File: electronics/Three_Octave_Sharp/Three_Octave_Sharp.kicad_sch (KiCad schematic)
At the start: 107 parts, among them J1 HRO_TYPE-C-31-M-12, SW1 Key Tab, SW10 Key O, SW11 Key P, SW12 Key BS, SW16 Key Caps, SW17 Key A, SW18 Key S, SW19 Key D, SW2 Key Q, SW20 Key F, SW21 Alps_Alpine_SKRP, SW21 Key G, SW22 Alps_Alpine_SKRP, SW22 Key H, SW23 Key J, SW24 Key K, SW25 Key L, SW26 Key Return, SW3 Key W, SW30 Key Shift, SW31 Key Z, SW32 Key X, SW33 Key C, SW33 Key Shift, SW34 Key V, SW35 Key B, SW36 Key N, SW37 Key M, SW38 Key ,, SW4 Key E, SW43 Key Ctrl, SW44 Key Cmd, SW45 Key Space, SW46 Key Opt, SW47 Key Fn, SW5 Key R, SW6 Key T, SW7 Key Y, SW8 Key U, SW9 Key I, U1 AP2112K-3.3, U2 Raspberry_Pi_RP2040, U2 W25Q64JVXGIQ, Y1 12MHz

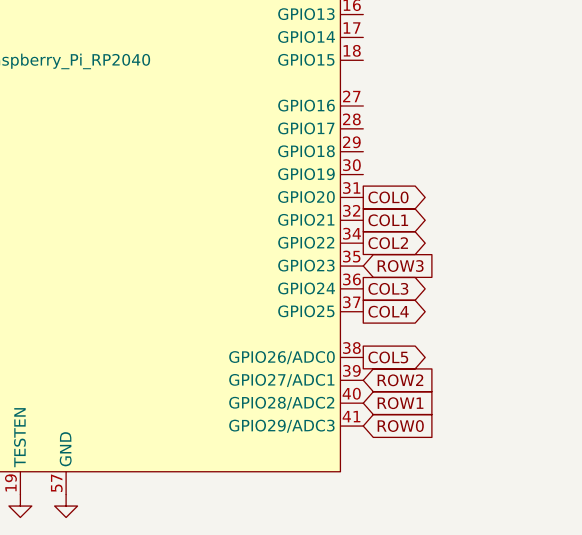
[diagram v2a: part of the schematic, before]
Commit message: WIP: Update PCB design
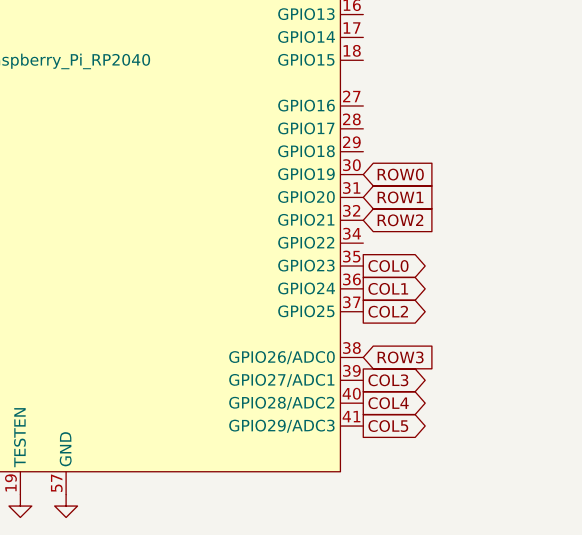
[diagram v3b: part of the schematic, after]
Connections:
- net COL0: now also U2.35 (GPIO23); no longer U2.31 (GPIO20)
- net COL1: now also U2.36 (GPIO24); no longer U2.32 (GPIO21)
- net COL2: now also U2.37 (GPIO25); no longer U2.34 (GPIO22)
- net COL3: now also U2.39 (GPIO27/ADC1); no longer U2.36 (GPIO24)
- net COL4: now also U2.40 (GPIO28/ADC2); no longer U2.37 (GPIO25)
- net COL5: now also U2.41 (GPIO29/ADC3); no longer U2.38 (GPIO26/ADC0)
- net ROW0: now also U2.30 (GPIO19); no longer U2.41 (GPIO29/ADC3)
- net ROW1: now also U2.31 (GPIO20); no longer U2.40 (GPIO28/ADC2)
- net ROW2: now also U2.32 (GPIO21); no longer U2.39 (GPIO27/ADC1)
- net ROW3: now also U2.38 (GPIO26/ADC0); no longer U2.35 (GPIO23)
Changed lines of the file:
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@@
     )
   )
-  (global_label "COL4" (shape output) (at 161.925 256.54 0) (fields_autoplaced)
+  (global_label "COL4" (shape output) (at 161.925 266.7 0) (fields_autoplaced)
+    (effects (font (size 1.27 1.27)) (justify left))
+    (property "Intersheetrefs" "${INTERSHEET_REFS}" (at 169.7483 266.7 0)
+      (effects (font (size 1.27 1.27)) (justify left) hide)
+    )
+  )
+  (global_label "COL6" (shape output) (at 161.925 187.96 0) (fields_autoplaced)
+    (effects (font (size 1.27 1.27)) (justify left))
+    (property "Intersheetrefs" "${INTERSHEET_REFS}" (at 169.7483 187.96 0)
+      (effects (font (size 1.27 1.27)) (justify left) hide)
+    )
+  )
+  (global_label "ROW3" (shape input) (at 161.925 261.62 0) (fields_autoplaced)
+    (effects (font (size 1.27 1.27)) (justify left))
+    (property "Intersheetrefs" "${INTERSHEET_REFS}" (at 170.1716 261.62 0)
+      (effects (font (size 1.27 1.27)) (justify left) hide)
+    )
+  )
+  (global_label "ROW3" (shape input) (at 30.48 104.14 180) (fields_autoplaced)
+    (effects (font (size 1.27 1.27)) (justify right))
+    (property "Intersheetrefs" "${INTERSHEET_REFS}" (at 22.2334 104.14 0)
+      (effects (font (size 1.27 1.27)) (justify right) hide)
+    )
+  )
+  (global_label "ROW2" (shape input) (at 161.925 246.38 0) (fields_autoplaced)
+    (effects (font (size 1.27 1.27)) (justify left))
+    (property "Intersheetrefs" "${INTERSHEET_REFS}" (at 170.1716 246.38 0)
+      (effects (font (size 1.27 1.27)) (justify left) hide)
+    )
+  )
+  (global_label "~{USB_BOOT}" (shape input) (at 34.925 241.3 180) (fields_autoplaced)
+    (effects (font (size 1.27 1.27)) (justify right))
+    (property "Intersheetrefs" "${INTERSHEET_REFS}" (at 22.8357 241.2206 0)
+      (effects (font (size 1.27 1.27)) (justify right) hide)
+    )
+  )
+  (global_label "COL8" (shape output) (at 161.925 193.04 0) (fields_autoplaced)
+    (effects (font (size 1.27 1.27)) (justify left))
+    (property "Intersheetrefs" "${INTERSHEET_REFS}" (at 169.7483 193.04 0)
+      (effects (font (size 1.27 1.27)) (justify left) hide)
+    )
+  )
+  (global_label "D+" (shape input) (at 62.865 152.4 0) (fields_autoplaced)
+    (effects (font (size 1.27 1.27)) (justify left))
+    (property "Intersheetrefs" "${INTERSHEET_REFS}" (at 68.1205 152.3206 0)
+      (effects (font (size 1.27 1.27)) (justify left) hide)
+    )
+  )
+  (global_label "COL2" (shape output) (at 161.925 256.54 0) (fields_autoplaced)
     (effects (font (size 1.27 1.27)) (justify left))
     (property "Intersheetrefs" "${INTERSHEET_REFS}" (at 169.7483 256.54 0)
@@
     )
   )
-  (global_label "COL6" (shape output) (at 161.925 187.96 0) (fields_autoplaced)
-    (effects (font (size 1.27 1.27)) (justify left))
-    (property "Intersheetrefs" "${INTERSHEET_REFS}" (at 169.7483 187.96 0)
-      (effects (font (size 1.27 1.27)) (justify left) hide)
-    )
-  )
-  (global_label "ROW3" (shape input) (at 161.925 251.46 0) (fields_autoplaced)
-    (effects (font (size 1.27 1.27)) (justify left))
-    (property "Intersheetrefs" "${INTERSHEET_REFS}" (at 170.1716 251.46 0)
-      (effects (font (size 1.27 1.27)) (justify left) hide)
-    )
-  )
-  (global_label "ROW3" (shape input) (at 30.48 104.14 180) (fields_autoplaced)
-    (effects (font (size 1.27 1.27)) (justify right))
-    (property "Intersheetrefs" "${INTERSHEET_REFS}" (at 22.2334 104.14 0)
-      (effects (font (size 1.27 1.27)) (justify right) hide)
-    )
-  )
-  (global_label "ROW2" (shape input) (at 161.925 264.16 0) (fields_autoplaced)
-    (effects (font (size 1.27 1.27)) (justify left))
-    (property "Intersheetrefs" "${INTERSHEET_REFS}" (at 170.1716 264.16 0)
-      (effects (font (size 1.27 1.27)) (justify left) hide)
-    )
-  )
-  (global_label "~{USB_BOOT}" (shape input) (at 34.925 241.3 180) (fields_autoplaced)
-    (effects (font (size 1.27 1.27)) (justify right))
-    (property "Intersheetrefs" "${INTERSHEET_REFS}" (at 22.8357 241.2206 0)
-      (effects (font (size 1.27 1.27)) (justify right) hide)
-    )
-  )
-  (global_label "COL8" (shape output) (at 161.925 193.04 0) (fields_autoplaced)
-    (effects (font (size 1.27 1.27)) (justify left))
-    (property "Intersheetrefs" "${INTERSHEET_REFS}" (at 169.7483 193.04 0)
-      (effects (font (size 1.27 1.27)) (justify left) hide)
-    )
-  )
-  (global_label "D+" (shape input) (at 62.865 152.4 0) (fields_autoplaced)
-    (effects (font (size 1.27 1.27)) (justify left))
-    (property "Intersheetrefs" "${INTERSHEET_REFS}" (at 68.1205 152.3206 0)
-      (effects (font (size 1.27 1.27)) (justify left) hide)
-    )
-  )
-  (global_label "COL2" (shape output) (at 161.925 248.92 0) (fields_autoplaced)
-    (effects (font (size 1.27 1.27)) (justify left))
-    (property "Intersheetrefs" "${INTERSHEET_REFS}" (at 169.7483 248.92 0)
-      (effects (font (size 1.27 1.27)) (justify left) hide)
-    )
-  )
   (global_label "D-" (shape input) (at 95.885 259.08 180) (fields_autoplaced)
     (effects (font (size 1.27 1.27)) (justify right))
@@
     )
   )
-  (global_label "COL1" (shape output) (at 161.925 246.38 0) (fields_autoplaced)
-    (effects (font (size 1.27 1.27)) (justify left))
-    (property "Intersheetrefs" "${INTERSHEET_REFS}" (at 169.7483 246.38 0)
-      (effects (font (size 1.27 1.27)) (justify left) hide)
-    )
-  )
-  (global_label "COL5" (shape output) (at 161.925 261.62 0) (fields_autoplaced)
-    (effects (font (size 1.27 1.27)) (justify left))
-    (property "Intersheetrefs" "${INTERSHEET_REFS}" (at 169.7483 261.62 0)
+  (global_label "COL1" (shape output) (at 161.925 254 0) (fields_autoplaced)
+    (effects (font (size 1.27 1.27)) (justify left))
+    (property "Intersheetrefs" "${INTERSHEET_REFS}" (at 169.7483 254 0)
+      (effects (font (size 1.27 1.27)) (justify left) hide)
+    )
+  )
+  (global_label "COL5" (shape output) (at 161.925 269.24 0) (fields_autoplaced)
+    (effects (font (size 1.27 1.27)) (justify left))
+    (property "Intersheetrefs" "${INTERSHEET_REFS}" (at 169.7483 269.24 0)
       (effects (font (size 1.27 1.27)) (justify left) hide)
     )
@@
     )
   )
-  (global_label "COL3" (shape output) (at 161.925 254 0) (fields_autoplaced)
-    (effects (font (size 1.27 1.27)) (justify left))
-    (property "Intersheetrefs" "${INTERSHEET_REFS}" (at 169.7483 254 0)
+  (global_label "COL3" (shape output) (at 161.925 264.16 0) (fields_autoplaced)
+    (effects (font (size 1.27 1.27)) (justify left))
+    (property "Intersheetrefs" "${INTERSHEET_REFS}" (at 169.7483 264.16 0)
       (effects (font (size 1.27 1.27)) (justify left) hide)
     )
@@
     )
   )
-  (global_label "COL0" (shape output) (at 161.925 243.84 0) (fields_autoplaced)
-    (effects (font (size 1.27 1.27)) (justify left))
-    (property "Intersheetrefs" "${INTERSHEET_REFS}" (at 169.7483 243.84 0)
+  (global_label "COL0" (shape output) (at 161.925 251.46 0) (fields_autoplaced)
+    (effects (font (size 1.27 1.27)) (justify left))
+    (property "Intersheetrefs" "${INTERSHEET_REFS}" (at 169.7483 251.46 0)
       (effects (font (size 1.27 1.27)) (justify left) hide)
     )
@@
     )
   )
-  (global_label "ROW0" (shape input) (at 161.925 269.24 0) (fields_autoplaced)
-    (effects (font (size 1.27 1.27)) (justify left))
-    (property "Intersheetrefs" "${INTERSHEET_REFS}" (at 170.1716 269.24 0)
-      (effects (font (size 1.27 1.27)) (justify left) hide)
-    )
-  )
-  (global_label "ROW1" (shape input) (at 161.925 266.7 0) (fields_autoplaced)
-    (effects (font (size 1.27 1.27)) (justify left))
-    (property "Intersheetrefs" "${INTERSHEET_REFS}" (at 170.1716 266.7 0)
-      (effects (font (size 1.27 1.27)) (justify left) hide)
-    )
+  (global_label "ROW0" (shape input) (at 161.925 241.3 0) (fields_autoplaced)
+    (effects (font (size 1.27 1.27)) (justify left))
+    (property "Intersheetrefs" "${INTERSHEET_REFS}" (at 170.1716 241.3 0)
+      (effects (font (size 1.27 1.27)) (justify left) hide)
+    )
+  )
+  (global_label "ROW1" (shape input) (at 161.925 243.84 0) (fields_autoplaced)
+    (effects (font (size 1.27 1.27)) (justify left))
+    (property "Intersheetrefs" "${INTERSHEET_REFS}" (at 170.1716 243.84 0)
+      (effects (font (size 1.27 1.27)) (justify left) hide)
+    )

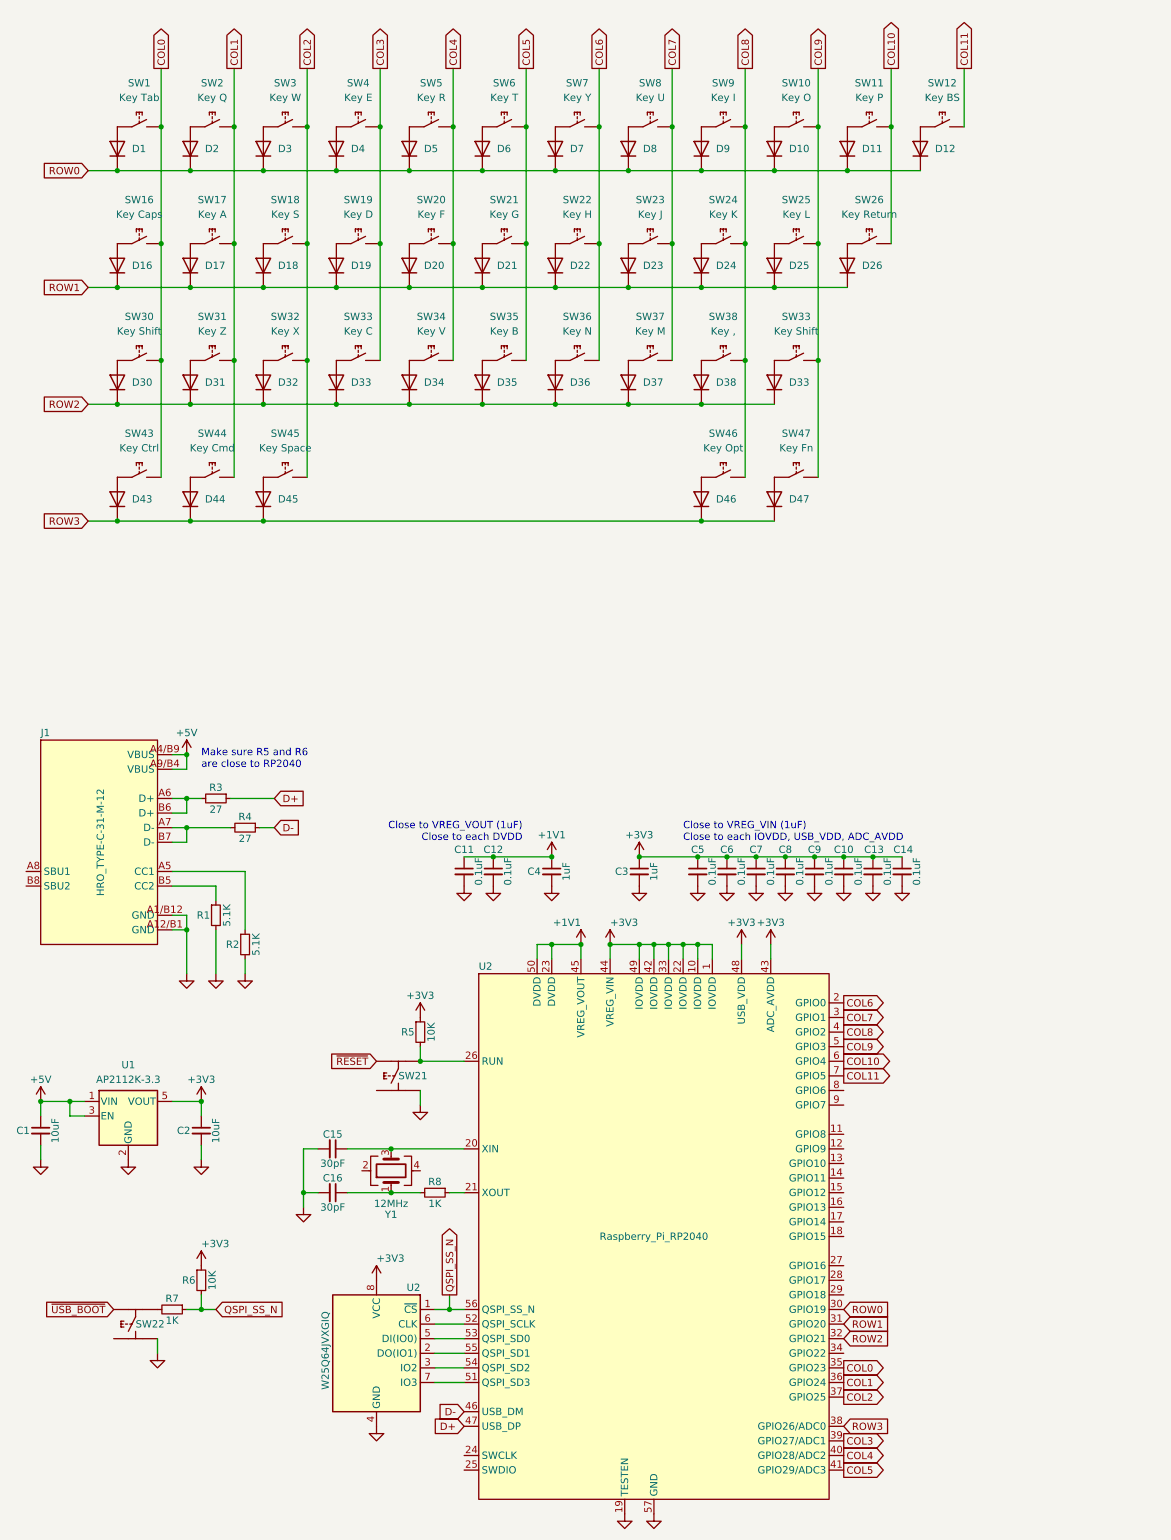
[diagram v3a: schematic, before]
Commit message: WIP: Update PCB design
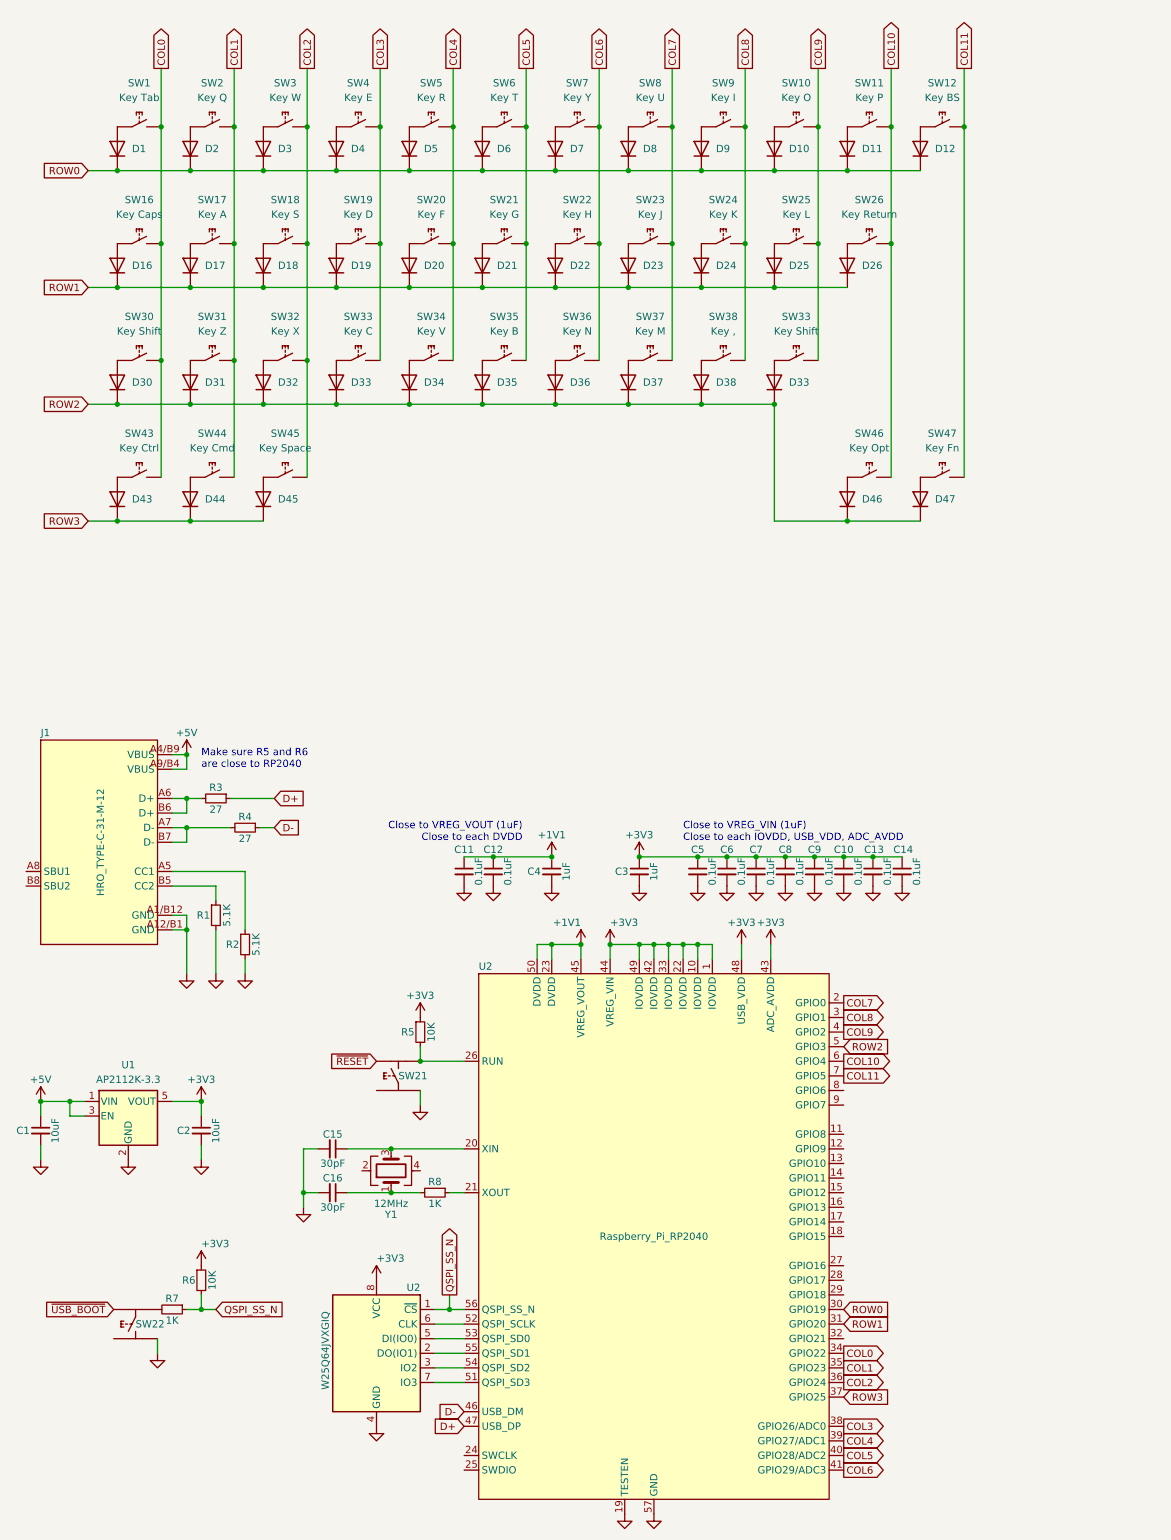
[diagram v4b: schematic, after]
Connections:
- net COL0: now also U2.34 (GPIO22); no longer U2.35 (GPIO23)
- net COL1: now also U2.35 (GPIO23); no longer U2.36 (GPIO24)
- net COL10: now also SW46.2
- net COL11: now also SW47.2
- net COL2: now also U2.36 (GPIO24); no longer U2.37 (GPIO25)
- net COL3: now also U2.38 (GPIO26/ADC0); no longer U2.39 (GPIO27/ADC1)
- net COL4: now also U2.39 (GPIO27/ADC1); no longer U2.40 (GPIO28/ADC2)
- net COL5: now also U2.40 (GPIO28/ADC2); no longer U2.41 (GPIO29/ADC3)
- net COL6: now also U2.41 (GPIO29/ADC3); no longer U2.2 (GPIO0)
- net COL7: now also U2.2 (GPIO0); no longer U2.3 (GPIO1)
- net COL8: now also U2.3 (GPIO1); no longer SW46.2, U2.4 (GPIO2)
- net COL9: now also U2.4 (GPIO2); no longer SW47.2, U2.5 (GPIO3)
- net GND: now also SW21.1; no longer SW21.3
- net ROW2: now also D46.1 (K), D47.1 (K), U2.5 (GPIO3); no longer U2.32 (GPIO21)
- net ROW3: now also U2.37 (GPIO25); no longer D46.1 (K), D47.1 (K), U2.38 (GPIO26/ADC0)
- net ~{RESET}: now also SW21.4; no longer SW21.2
- net at R5.2, U2.26 (RUN): now also SW21.3; no longer SW21.1
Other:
- moved on the sheet: D46, D47, SW21, SW46, SW47

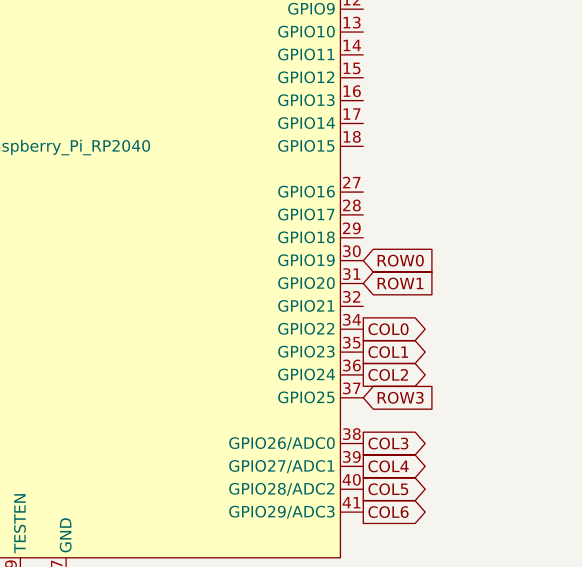
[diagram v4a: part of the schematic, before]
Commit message: WIP: Update PCB design
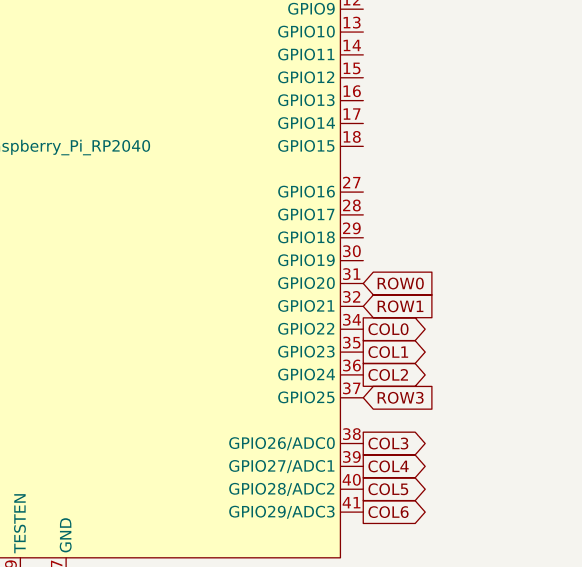
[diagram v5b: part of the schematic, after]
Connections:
- net ROW0: now also U2.31 (GPIO20); no longer U2.30 (GPIO19)
- net ROW1: now also U2.32 (GPIO21); no longer U2.31 (GPIO20)
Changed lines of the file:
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@@
     )
   )
-  (global_label "ROW0" (shape input) (at 161.925 241.3 0) (fields_autoplaced)
-    (effects (font (size 1.27 1.27)) (justify left))
-    (property "Intersheetrefs" "${INTERSHEET_REFS}" (at 170.1716 241.3 0)
-      (effects (font (size 1.27 1.27)) (justify left) hide)
-    )
-  )
-  (global_label "ROW1" (shape input) (at 161.925 243.84 0) (fields_autoplaced)
+  (global_label "ROW0" (shape input) (at 161.925 243.84 0) (fields_autoplaced)
     (effects (font (size 1.27 1.27)) (justify left))
     (property "Intersheetrefs" "${INTERSHEET_REFS}" (at 170.1716 243.84 0)
       (effects (font (size 1.27 1.27)) (justify left) hide)
     )
+  )
+  (global_label "ROW1" (shape input) (at 161.925 246.38 0) (fields_autoplaced)
+    (effects (font (size 1.27 1.27)) (justify left))
+    (property "Intersheetrefs" "${INTERSHEET_REFS}" (at 170.1716 246.38 0)
+      (effects (font (size 1.27 1.27)) (justify left) hide)
+    )
